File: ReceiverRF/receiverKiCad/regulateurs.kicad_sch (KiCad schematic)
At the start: 7 parts, among them J1 Conn_01x02, U2 AP2210N-3.3TRG1, U3 LP2980AIM5-5.0/NOPB

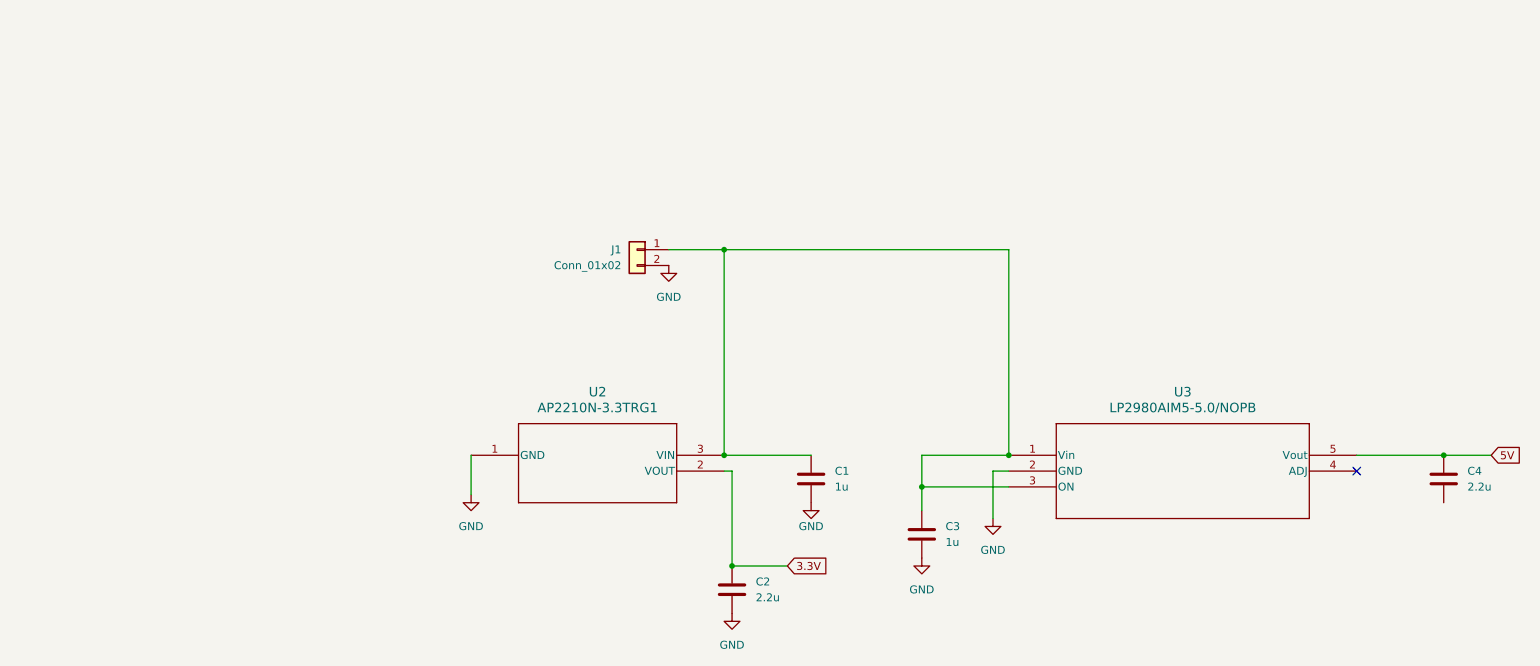
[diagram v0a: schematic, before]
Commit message: finir layout schematic et création projet firmware pour rfreceiver
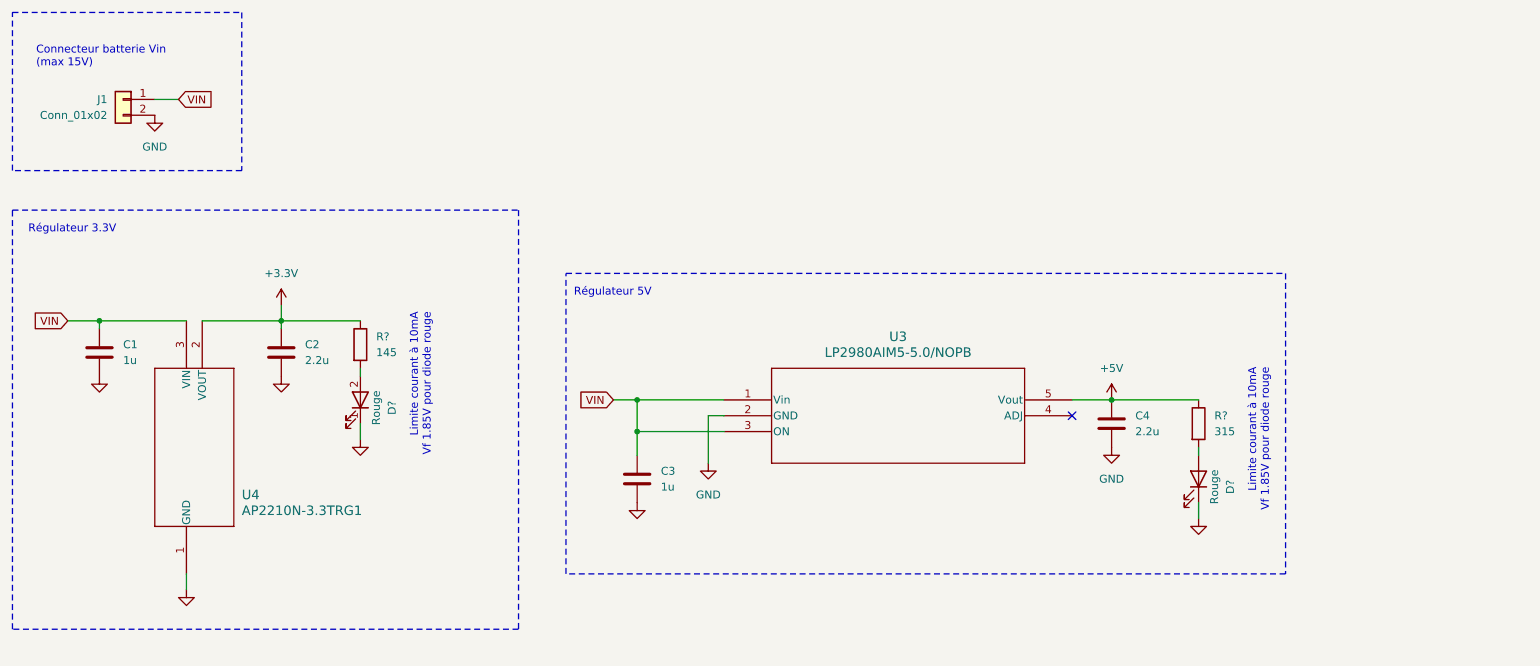
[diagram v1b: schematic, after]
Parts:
- added D? (x2): Rouge, footprint-receiver:LTST-C190EKT, symbol Device:LED
- added R?: 145, symbol Device:R
- added R?: 315, symbol Device:R
- renumbered U2 to U4
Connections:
- net GND: now also C4.2, D?.1 (K), D?.1 (K)
- net VIN: now reaches C1.1, C3.1, J1.1 (Pin_1), U3.1 (Vin), U3.3 (ON), U4.3 (VIN)
- net 3.3V renamed +3.3V
- net +3.3V: now also R?.1
- net 5V renamed +5V
- net +5V: now also R?.1
- new net: D?.2 (A), R?.2 (x2)
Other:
- note added: "Connecteur batterie Vin (max 15V)"
- note added: "Limite courant à 10mA Vf 1.85V pour diode rouge"
- note added: "Régulateur 3.3V"
- note added: "Régulateur 5V"
- moved on the sheet: C1, C2, C3, C4, J1, U3, U4
